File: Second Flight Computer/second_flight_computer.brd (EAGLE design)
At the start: 100 x 100 mm, 17 parts, among them J1 1X2-3.5MM, J2 1X2-3.5MM, J3 1X2-3.5MM, Q1 IRF540, Q2 IRF540, SW1 SPST_TACT-EVQQ2, U1 GY-521MPU6050

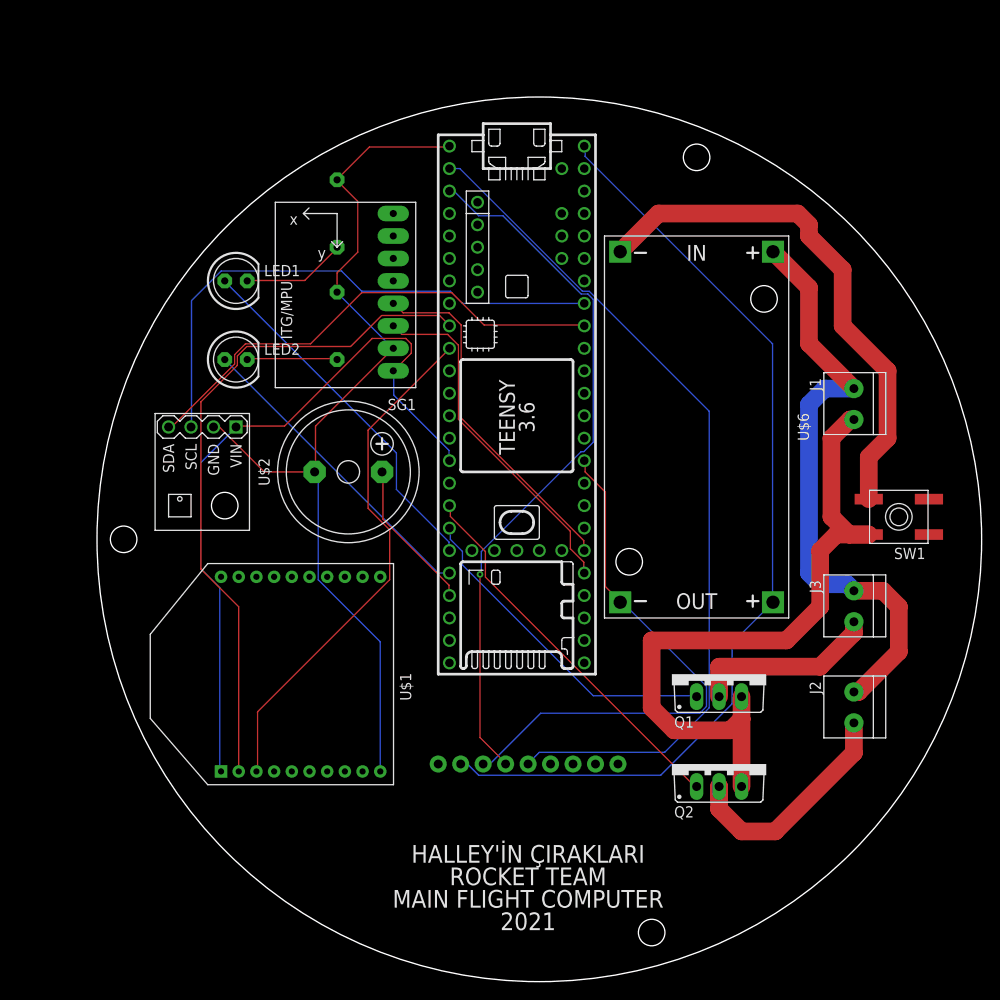
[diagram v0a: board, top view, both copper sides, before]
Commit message: Second Flight Computer
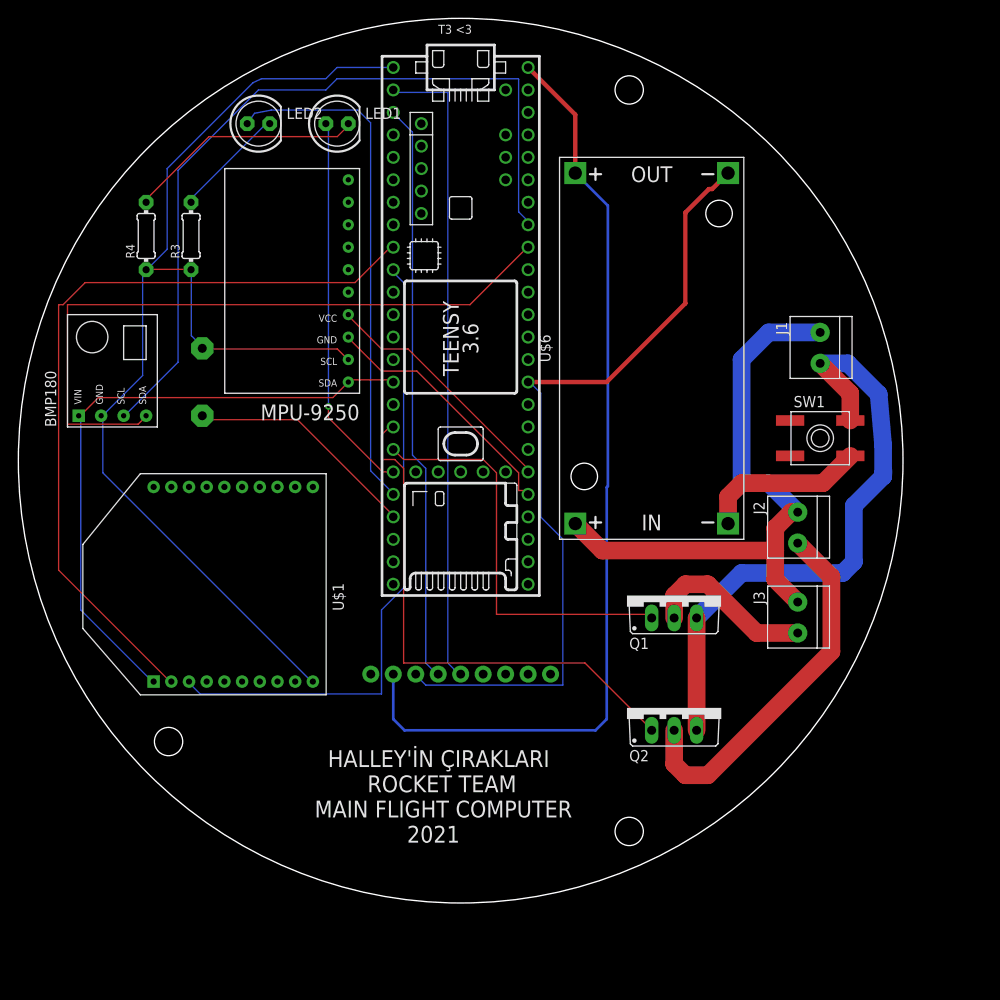
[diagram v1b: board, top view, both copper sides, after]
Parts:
- removed U$2: TEMP-HUM-PRES-BME280, diy-modules:TEMP-HUM-PRES-BME280
- removed U1: GY-521MPU6050, gy-521:GY-521
- added BMP1: BMP180, BMP180-Lib:BMP180
- added MPU-1: MPU-9250, MPU-9250:MPU-9250
- moved LED2 26.8 mm to (21.6, 77.5)
- moved R4 21.7 mm to (8.89, 64.8), flipped to the top, turned to 90 degrees
- moved J2 21.3 mm to (82.5, 31.8)
- moved LED1 21.1 mm to (30.5, 77.5)
- moved R3 19.4 mm to (14.0, 64.8), flipped to the top, turned to 90 degrees
- moved SG1 19.4 mm to (15.2, 48.3), flipped to the bottom, turned to 270 degrees
- moved U$5 12.7 mm to (41.9, 27.9)
- moved U$1 12.7 mm to (15.2, 25.4)
- moved SW1 12.6 mm to (85.1, 41.9), turned to 0 degrees
- moved U$3 10.9 mm to (44.5, 55.9)
- moved U$6 10.2 mm to (66.0, 52.1), turned to 90 degrees
- moved Q1 10.2 mm to (68.6, 24.1)
- moved Q2 8.13 mm to (68.6, 11.4)
- moved J1 7.41 mm to (85.1, 52.1)
- moved J3 6.48 mm to (82.5, 21.6)
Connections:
- net 3.3V: now also BMP1.VIN, MPU-1.VCC; no longer U$2.1, U1.VCC
- net GND: now also BMP1.GND, MPU-1.GND; no longer U$2.2, U1.GND
- net SCL0: now also BMP1.SCL; no longer U$2.3
- net SCL1: now also MPU-1.SCL; no longer U1.SCL
- net SDA0: now also BMP1.SDA; no longer U$2.4
- net SDA1: now also MPU-1.SDA; no longer U1.SDA
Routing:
- net IN-: track 59.2 -> 18.8 mm
- net GND2: track 61.7 -> 91.5 mm
- net SCL0: track 61.6 -> 90.0 mm
- net GND: track 106.2 -> 133.2 mm
- net GPSTX: track 97.4 -> 72.8 mm
- net LED2: track 35.4 -> 58.2 mm
- net SDA0: track 55.5 -> 77.6 mm
- net RELAY1: track 43.6 -> 60.6 mm
- net N$1: track 11.8 -> 26.8 mm
- net GPSRX: track 80.5 -> 65.6 mm, vias 1 -> 0
- net RECOVERY1-: track 27.2 -> 41.8 mm
- net RFRX: track 58.9 -> 71.8 mm
- net SDA1: track 39.9 -> 27.9 mm
- net 3.3V: track 82.6 -> 70.9 mm
- net RFTX: track 76.8 -> 88.5 mm
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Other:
- board text added: "HALLEY'İN ÇIRAKLARI ROCKET TEAM MAIN FLIGHT COMPUTER 2021"
- board text added: "T3 <3"
- board text removed: "2021"
- board text removed: "HALLEY'İN ÇIRAKLARI"
- board text removed: "MAIN FLIGHT COMPUTER"
- board text removed: "ROCKET TEAM"
